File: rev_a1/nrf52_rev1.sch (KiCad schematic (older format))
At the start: 27 parts, among them P1 CONN_01X18, P2 CONN_01X18, P3 USB_OTG, U1 nRF52832, U2 CP2102, U3 LT1129CST-3.3, Y1 32K, Y2 32M

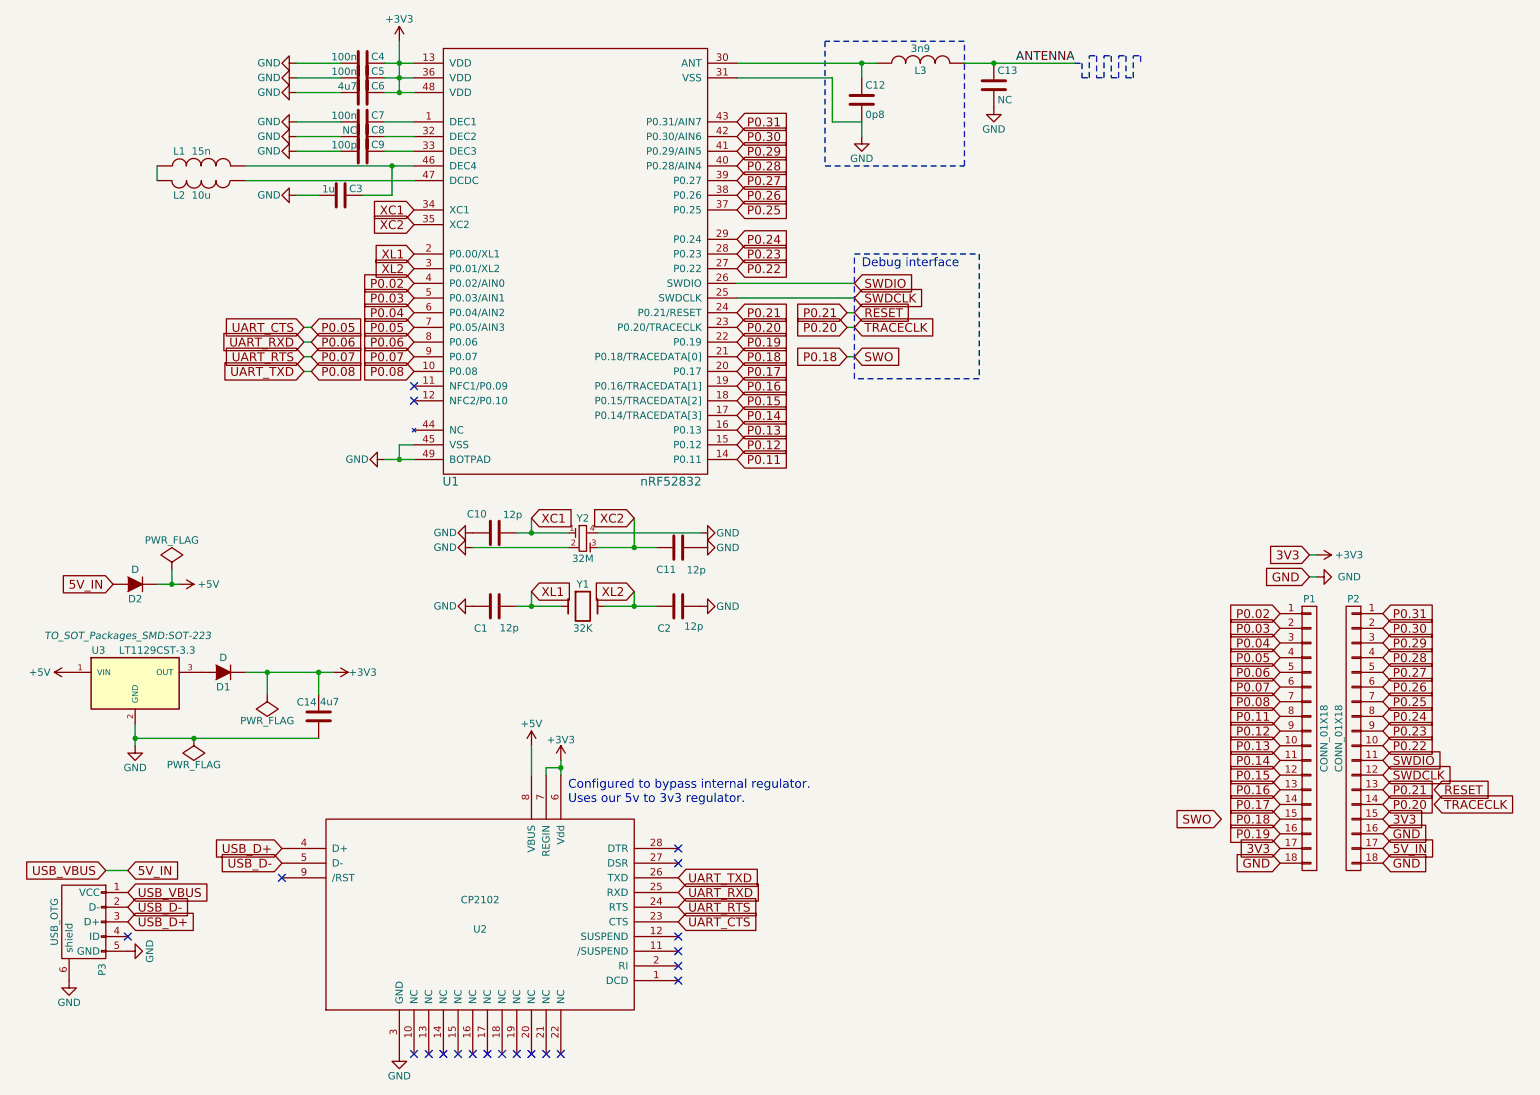
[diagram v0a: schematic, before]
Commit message: WIP
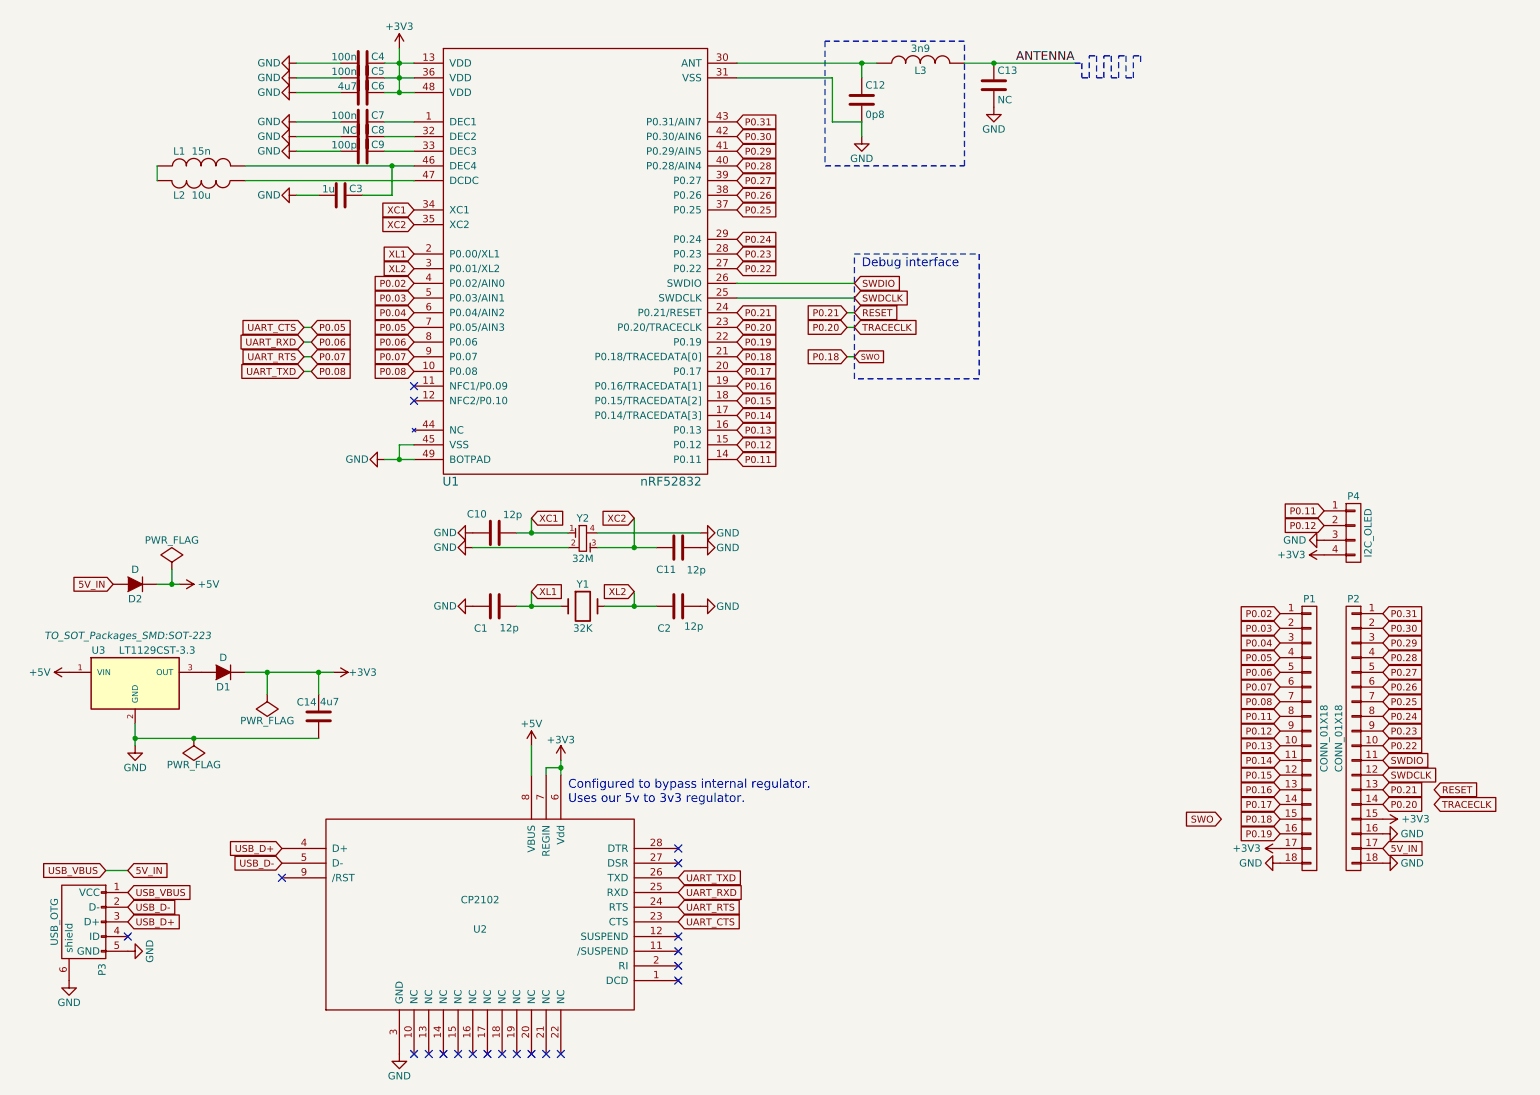
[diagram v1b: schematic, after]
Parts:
- added P4: I2C_OLED, Socket_Strips:Socket_Strip_Straight_1x04, symbol CONN_01X04
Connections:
- net +3V3: now also P4.4 (P4)
- net GND: now also P4.3 (P3)
- net P0.11: now also P4.1 (P1)
- net P0.12: now also P4.2 (P2)

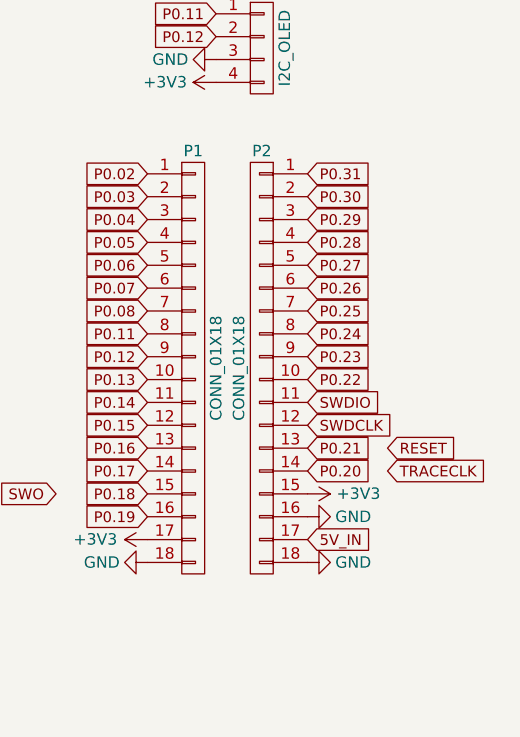
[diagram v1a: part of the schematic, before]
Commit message: WIP
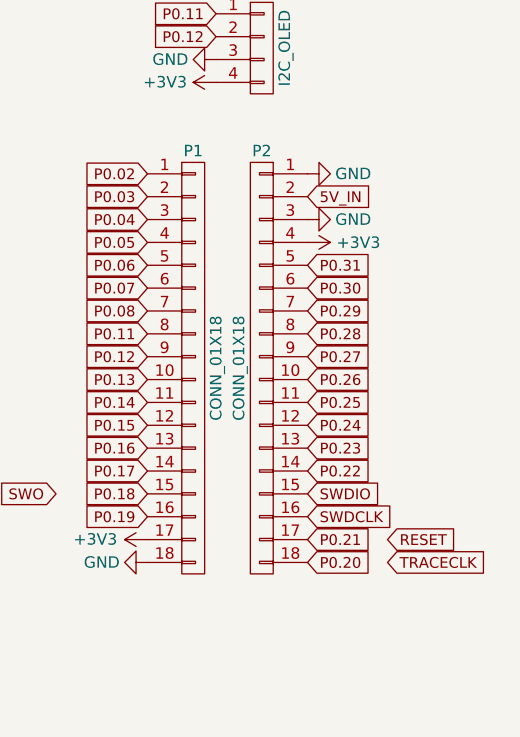
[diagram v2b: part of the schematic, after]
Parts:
- C1, C10, C11, C12, C13, C14, C2, C3, C4, C5, C6, C7, C8, C9: footprint RuuviTag:0402_CAP -> RuuviTag:0603_CAP
- L1, L3: footprint RuuviTag:0402_IND -> RuuviTag:0603_IND
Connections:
- net +3V3: now also P2.4 (P4); no longer P2.15 (P15)
- net 5V_IN: now also P2.2 (P2); no longer P2.17 (P17)
- net GND: now also P2.1 (P1), P2.3 (P3); no longer P2.16 (P16), P2.18 (P18)
- net P0.20: now also P2.18 (P18); no longer P2.14 (P14)
- net P0.21: now also P2.17 (P17); no longer P2.13 (P13)
- net P0.22: now also P2.14 (P14); no longer P2.10 (P10)
- net P0.23: now also P2.13 (P13); no longer P2.9 (P9)
- net P0.24: now also P2.12 (P12); no longer P2.8 (P8)
- net P0.25: now also P2.11 (P11); no longer P2.7 (P7)
- net P0.26: now also P2.10 (P10); no longer P2.6 (P6)
- net P0.27: now also P2.9 (P9); no longer P2.5 (P5)
- net P0.28: now also P2.8 (P8); no longer P2.4 (P4)
- net P0.29: now also P2.7 (P7); no longer P2.3 (P3)
- net P0.30: now also P2.6 (P6); no longer P2.2 (P2)
- net P0.31: now also P2.5 (P5); no longer P2.1 (P1)
- net SWDCLK: now also P2.16 (P16); no longer P2.12 (P12)
- net SWDIO: now also P2.15 (P15); no longer P2.11 (P11)
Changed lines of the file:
@@
 F 0 "C4" V 2855 858 50  0000 L CNN
 F 1 "100n" V 2828 761 50  0000 R TNN
-F 2 "RuuviTag:0402_CAP" H 2938 650 50  0001 C CNN
+F 2 "RuuviTag:0603_CAP" H 2938 650 50  0001 C CNN
 F 3 "" H 2900 800 50  0000 C CNN
 	1    2900 800
@@
 F 0 "C5" V 2855 958 50  0000 L CNN
 F 1 "100n" V 2828 861 50  0000 R TNN
-F 2 "RuuviTag:0402_CAP" H 2938 750 50  0001 C CNN
+F 2 "RuuviTag:0603_CAP" H 2938 750 50  0001 C CNN
 F 3 "" H 2900 900 50  0000 C CNN
 	1    2900 900
@@
 F 0 "C6" V 2855 1058 50  0000 L CNN
 F 1 "4u7" V 2828 961 50  0000 R TNN
-F 2 "RuuviTag:0402_CAP" H 2938 850 50  0001 C CNN
+F 2 "RuuviTag:0603_CAP" H 2938 850 50  0001 C CNN
 F 3 "" H 2900 1000 50  0000 C CNN
 	1    2900 1000
@@
 F 0 "C7" V 2855 1258 50  0000 L CNN
 F 1 "100n" V 2828 1161 50  0000 R TNN
-F 2 "RuuviTag:0402_CAP" H 2938 1050 50  0001 C CNN
+F 2 "RuuviTag:0603_CAP" H 2938 1050 50  0001 C CNN
 F 3 "" H 2900 1200 50  0000 C CNN
 	1    2900 1200
@@
 F 0 "C8" V 2855 1358 50  0000 L CNN
 F 1 "NC" V 2828 1261 50  0000 R TNN
-F 2 "RuuviTag:0402_CAP" H 2938 1150 50  0001 C CNN
+F 2 "RuuviTag:0603_CAP" H 2938 1150 50  0001 C CNN
 F 3 "" H 2900 1300 50  0000 C CNN
 	1    2900 1300
@@
 F 0 "C9" V 2855 1458 50  0000 L CNN
 F 1 "100p" V 2828 1361 50  0000 R TNN
-F 2 "RuuviTag:0402_CAP" H 2938 1250 50  0001 C CNN
+F 2 "RuuviTag:0603_CAP" H 2938 1250 50  0001 C CNN
 F 3 "" H 2900 1400 50  0000 C CNN
 	1    2900 1400
@@
 F 0 "L1" V 1900 1650 50  0000 C CNN
 F 1 "15n" V 1900 1500 50  0000 C CNN
-F 2 "RuuviTag:0402_IND" H 1800 1500 50  0001 C CNN
+F 2 "RuuviTag:0603_IND" H 1800 1500 50  0001 C CNN
 F 3 "" H 1800 1500 50  0000 C CNN
 	1    1800 1500
@@
 F 0 "C3" V 2705 1758 50  0000 L CNN
 F 1 "1u" V 2678 1661 50  0000 R TNN
-F 2 "RuuviTag:0402_CAP" H 2788 1550 50  0001 C CNN
+F 2 "RuuviTag:0603_CAP" H 2788 1550 50  0001 C CNN
 F 3 "" H 2750 1700 50  0000 C CNN
 	1    2750 1700
@@
 F 0 "C10" V 3672 3810 50  0000 L CNN
 F 1 "12p" V 3647 4187 50  0000 R TNN
-F 2 "RuuviTag:0402_CAP" H 3838 3850 50  0001 C CNN
+F 2 "RuuviTag:0603_CAP" H 3838 3850 50  0001 C CNN
 F 3 "" H 3800 4000 50  0000 C CNN
 	1    3800 4000
@@
 F 0 "C11" V 5200 3950 50  0000 L CNN
 F 1 "12p" V 5174 4288 50  0000 R TNN
-F 2 "RuuviTag:0402_CAP" H 5088 3950 50  0001 C CNN
+F 2 "RuuviTag:0603_CAP" H 5088 3950 50  0001 C CNN
 F 3 "" H 5050 4100 50  0000 C CNN
 	1    5050 4100
@@
 F 0 "C12" H 6325 1150 50  0000 L CNN
 F 1 "0p8" H 6325 950 50  0000 L CNN
-F 2 "RuuviTag:0402_CAP" H 6338 900 50  0001 C CNN
+F 2 "RuuviTag:0603_CAP" H 6338 900 50  0001 C CNN
 F 3 "" H 6300 1050 50  0000 C CNN
 	1    6300 1050
@@
 F 0 "L3" V 6650 800 50  0000 C CNN
 F 1 "3n9" V 6800 800 50  0000 C CNN
-F 2 "RuuviTag:0402_IND" H 6700 800 50  0001 C CNN
+F 2 "RuuviTag:0603_IND" H 6700 800 50  0001 C CNN
 F 3 "" H 6700 800 50  0000 C CNN
 	1    6700 800
@@
 F 0 "C13" H 7225 1050 50  0000 L CNN
 F 1 "NC" H 7225 850 50  0000 L CNN
-F 2 "RuuviTag:0402_CAP" H 7238 800 50  0001 C CNN
+F 2 "RuuviTag:0603_CAP" H 7238 800 50  0001 C CNN
 F 3 "" H 7200 950 50  0000 C CNN
 	1    7200 950
@@
 	1    0    0    -1
 $EndComp
-Text GLabel 9850 6150 2    47   Input ~ 0
+Text GLabel 9850 4650 2    47   Input ~ 0
 5V_IN
 $Comp
@@
 Text GLabel 9150 6050 0    47   Input ~ 0
 P0.19
+Text GLabel 9850 6250 2    47   Input ~ 0
+P0.20
+Text GLabel 9850 6150 2    47   Input ~ 0
+P0.21
 Text GLabel 9850 5850 2    47   Input ~ 0
-P0.20
+P0.22
 Text GLabel 9850 5750 2    47   Input ~ 0
-P0.21
+P0.23
+Text GLabel 9850 5650 2    47   Input ~ 0
+P0.24
+Text GLabel 9850 5550 2    47   Input ~ 0
+P0.25
 Text GLabel 9850 5450 2    47   Input ~ 0
-P0.22
+P0.26
 Text GLabel 9850 5350 2    47   Input ~ 0
-P0.23
+P0.27
 Text GLabel 9850 5250 2    47   Input ~ 0
-P0.24
+P0.28
 Text GLabel 9850 5150 2    47   Input ~ 0
-P0.25
+P0.29
 Text GLabel 9850 5050 2    47   Input ~ 0
-P0.26
-Text GLabel 9850 4950 2    47   Input ~ 0
-P0.27
-Text GLabel 9850 4850 2    47   Input ~ 0
-P0.28
-Text GLabel 9850 4750 2    47   Input ~ 0
-P0.29
-Text GLabel 9850 4650 2    47   Input ~ 0
 P0.30
 Text GLabel 9150 5950 0    47   Input ~ 0
 P0.18
-Text GLabel 9850 4550 2    47   Input ~ 0
+Text GLabel 9850 4950 2    47   Input ~ 0
 P0.31
 Text GLabel 3250 2300 0    47   Input ~ 0
@@
 F 0 "C1" V 3650 4550 50  0000 L CNN
 F 1 "12p" V 3623 4467 50  0000 R TNN
-F 2 "RuuviTag:0402_CAP" H 3838 4350 50  0001 C CNN
+F 2 "RuuviTag:0603_CAP" H 3838 4350 50  0001 C CNN
 F 3 "" H 3800 4500 50  0000 C CNN
 	1    3800 4500
@@
 F 0 "C2" V 4900 4550 50  0000 L CNN
 F 1 "12p" V 4884 4460 50  0000 R TNN
-F 2 "RuuviTag:0402_CAP" H 5088 4350 50  0001 C CNN
+F 2 "RuuviTag:0603_CAP" H 5088 4350 50  0001 C CNN
 F 3 "" H 5050 4500 50  0000 C CNN
 	1    5050 4500
@@
 Text GLabel 3250 1900 0    47   Input ~ 0
 XC2
-Text GLabel 9850 5550 2    47   Input ~ 0
+Text GLabel 9850 5950 2    47   Input ~ 0
 SWDIO
-Text GLabel 9850 5650 2    47   Input ~ 0
+Text GLabel 9850 6050 2    47   Input ~ 0
 SWDCLK
 Text GLabel 6250 2500 2    47   Input ~ 0
@@
 F 0 "C14" H 2614 5153 50  0000 L CNN
 F 1 "4u7" H 2591 5180 50  0000 R TNN
-F 2 "RuuviTag:0402_CAP" H 2638 5100 50  0001 C CNN
+F 2 "RuuviTag:0603_CAP" H 2638 5100 50  0001 C CNN
 F 3 "" H 2600 5250 50  0000 C CNN
 	1    2600 5250
@@
 Wire Notes Line
 	7100 2950 6250 2950
-Text GLabel 10200 5850 2    47   Input ~ 0
+Text GLabel 10200 6250 2    47   Input ~ 0
 TRACECLK
-Text GLabel 10200 5750 2    47   Input ~ 0
+Text GLabel 10200 6150 2    47   Input ~ 0
 RESET
 Text GLabel 8750 5950 0    47   Input ~ 0
@@
 L GND #PWR032
 U 1 1 575DC996
-P 9850 6250
-F 0 "#PWR032" H 9850 6000 50  0001 C CNN
-F 1 "GND" V 9850 6050 50  0000 C CNN
-F 2 "" H 9850 6250 50  0000 C CNN
-F 3 "" H 9850 6250 50  0000 C CNN
-	1    9850 6250
-	0    -1   -1   0
+P 9850 4550
+F 0 "#PWR032" H 9850 4300 50  0001 C CNN
+F 1 "GND" V 9850 4350 50  0000 C CNN
+F 2 "" H 9850 4550 50  0000 C CNN
+F 3 "" H 9850 4550 50  0000 C CNN
+	1    9850 4550
+	0    -1   1    0
 $EndComp
 $Comp
 L +3V3 #PWR033
 U 1 1 575DCAE2
-P 9850 5950
-F 0 "#PWR033" H 9850 5800 50  0001 C CNN
-F 1 "+3V3" V 9849 6173 50  0000 C CNN
-F 2 "" H 9850 5950 50  0000 C CNN
-F 3 "" H 9850 5950 50  0000 C CNN
-	1    9850 5950
-	0    1    1    0
+P 9850 4850
+F 0 "#PWR033" H 9850 4700 50  0001 C CNN
+F 1 "+3V3" V 9849 5073 50  0000 C CNN
+F 2 "" H 9850 4850 50  0000 C CNN
+F 3 "" H 9850 4850 50  0000 C CNN
+	1    9850 4850
+	0    1    -1   0
 $EndComp
 $Comp
 L GND #PWR034
 U 1 1 575DCBF4
-P 9850 6050
-F 0 "#PWR034" H 9850 5800 50  0001 C CNN
-F 1 "GND" V 9850 5850 50  0000 C CNN
-F 2 "" H 9850 6050 50  0000 C CNN
-F 3 "" H 9850 6050 50  0000 C CNN
-	1    9850 6050
-	0    -1   -1   0
-$EndComp
-$Comp
+P 9850 4750
+F 0 "#PWR034" H 9850 4500 50  0001 C CNN
+F 1 "GND" V 9850 4550 50  0000 C CNN
+F 2 "" H 9850 4750 50  0000 C CNN
+F 3 "" H 9850 4750 50  0000 C CNN
+	1    9850 4750
+	0    -1   1    0
+$EndComp
+$Comp
